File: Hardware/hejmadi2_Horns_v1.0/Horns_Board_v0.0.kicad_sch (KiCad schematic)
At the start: 4 parts, among them J1 Conn_01x03, J2 Conn_01x02, J3 Conn_01x02, J4 Conn_01x02

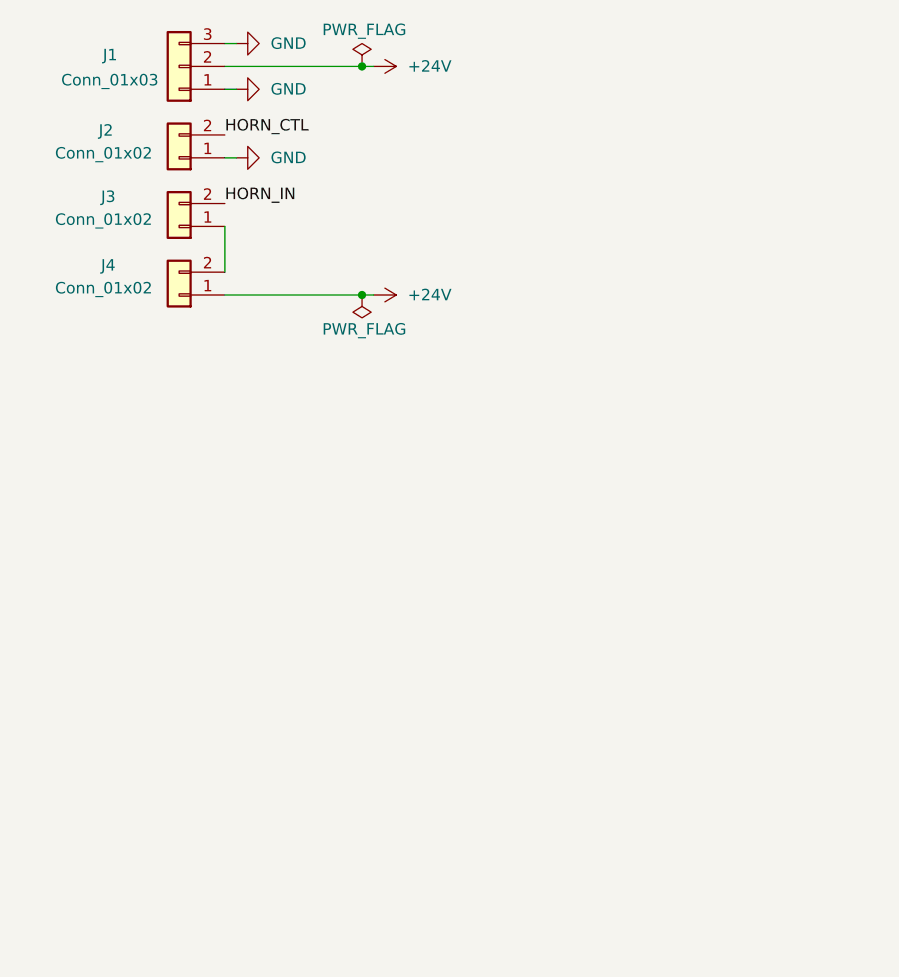
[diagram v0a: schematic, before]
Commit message: Horns Board schematic
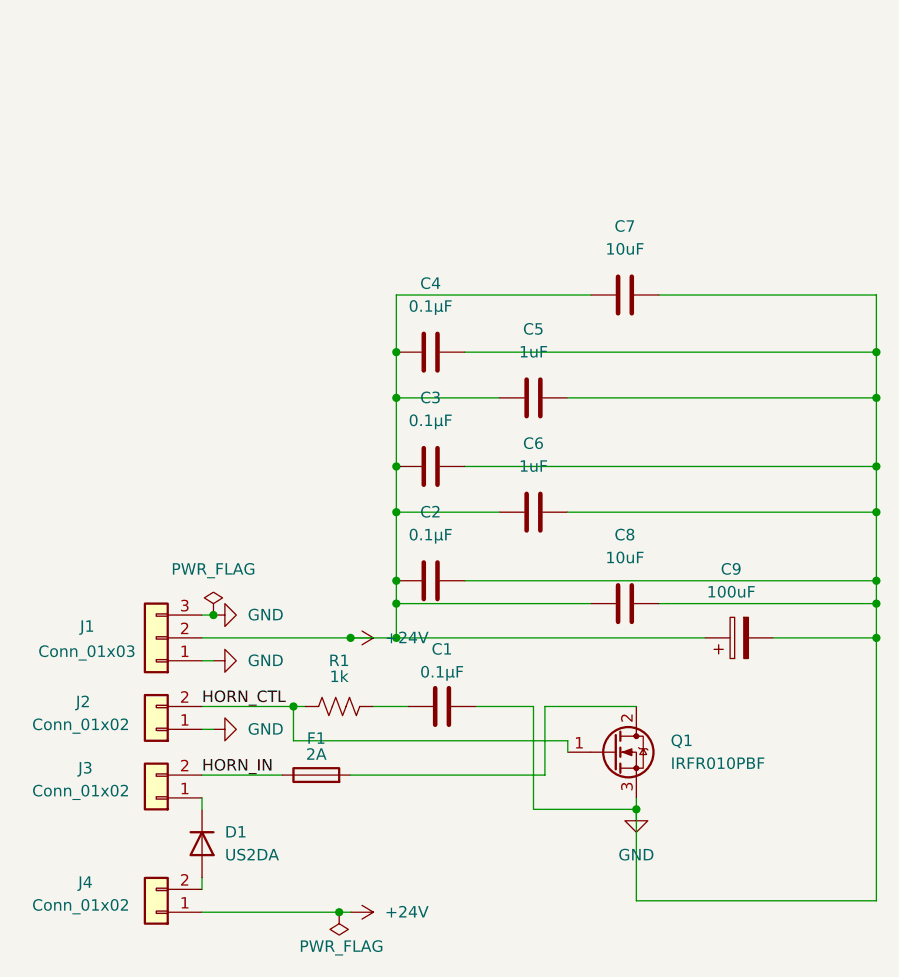
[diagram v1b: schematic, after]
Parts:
- added C1, C2, C3, C4: 0.1µF, symbol device:C
- added C5, C6: 1uF, symbol device:C
- added C7, C8: 10uF, symbol device:C
- added C9: 100uF, symbol device:C_Polarized
- added D1: US2DA, Diode_SMD:D_SMA, symbol Diode:US2DA
- added F1: 2A, symbol device:Fuse
- added Q1: IRFR010PBF, symbol device:Q_NMOS_GDS
- added R1: 1k, symbol Device:R_US
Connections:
- net +24V: now also C2.1, C3.1, C4.1, C5.1, C6.1, C7.1, C8.1, C9.1
- net GND: now also C1.2, C2.2, C3.2, C4.2, C5.2, C6.2, C7.2, C8.2, C9.2, Q1.3 (S)
- net HORN_CTL: now also Q1.1 (G), R1.1
- net HORN_IN: now also F1.1
- net at J4.2 (Pin_2): now also D1.2 (A); no longer J3.1 (Pin_1)
- new net: C1.1, R1.2
- new net: D1.1 (K), J3.1 (Pin_1)
- new net: F1.2, Q1.2 (D)
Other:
- moved on the sheet: J1, J2, J3, J4
